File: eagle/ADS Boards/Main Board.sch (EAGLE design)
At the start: 14 parts

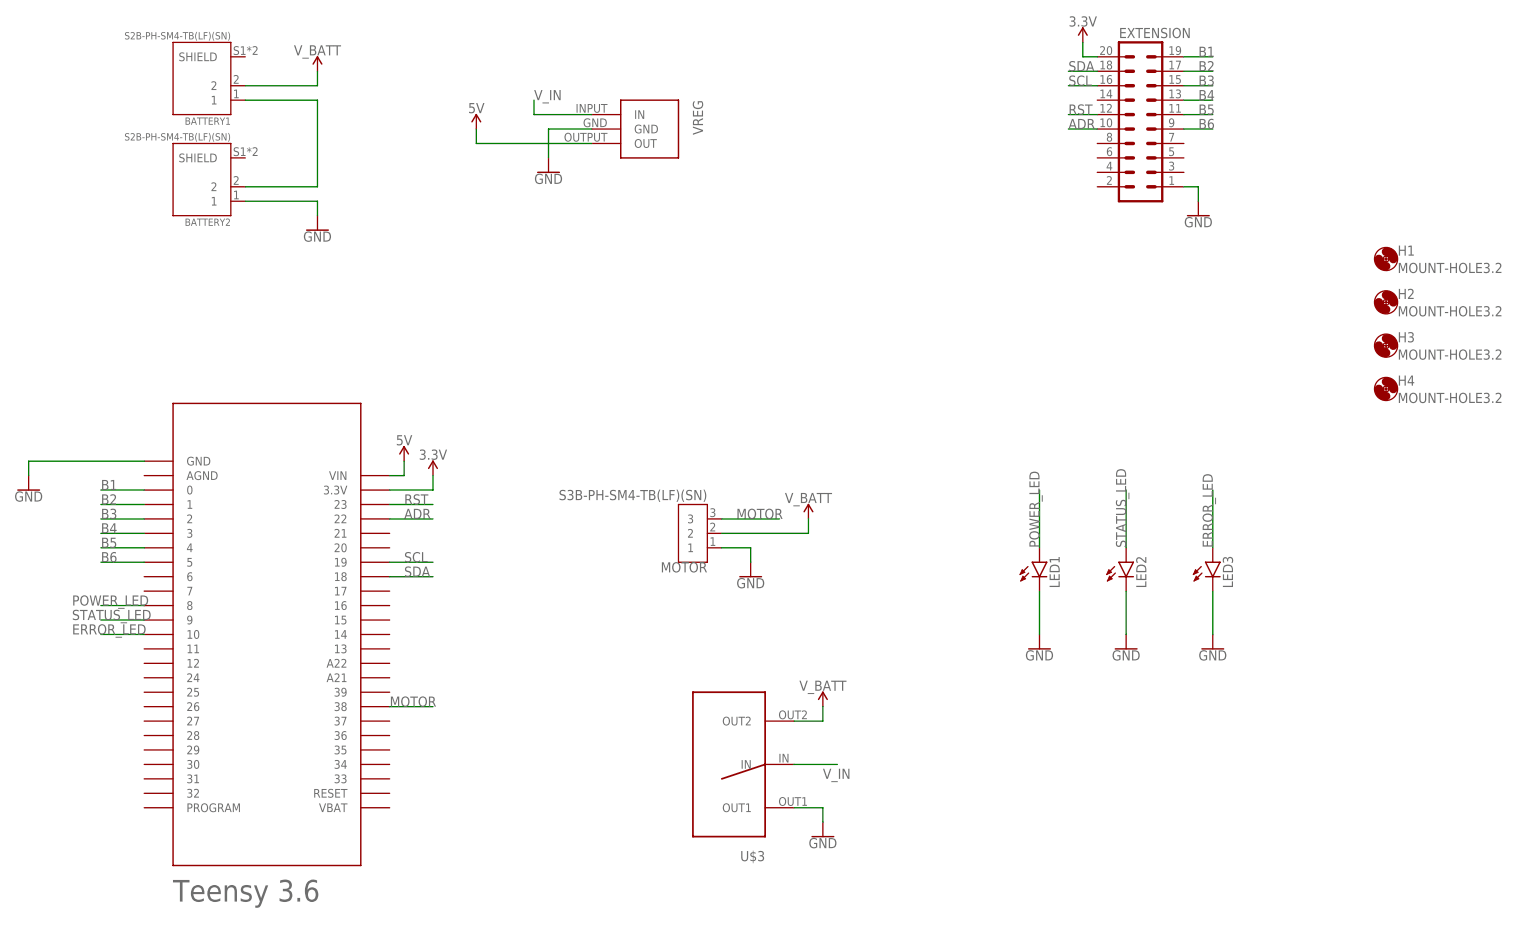
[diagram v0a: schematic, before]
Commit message: Finalized Boards, Gerbers, and DXF files.
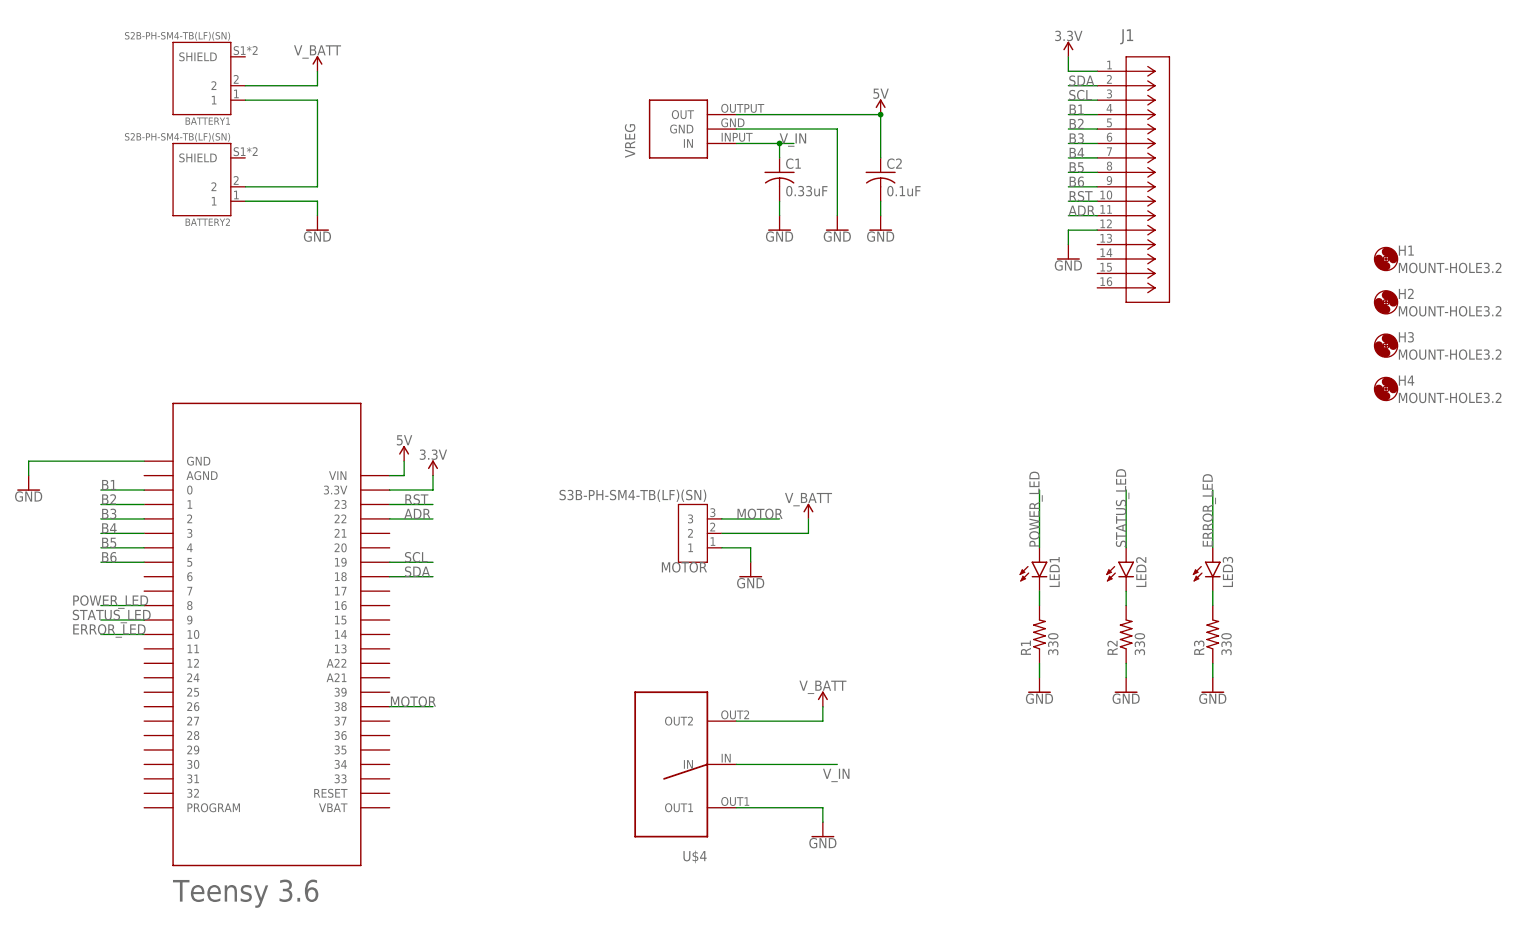
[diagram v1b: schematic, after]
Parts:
- removed EXTENSION: (no value), con-lstb:MA10-2
- removed U$3: SLIDE_SWITCH, ME433:SLIDE_SWITCH
- added C1: 0.33uF, resistor:C-USC0805
- added C2: 0.1uF, resistor:C-USC0805
- added J1: 62674-121121ALF, NUSTARS ADS Library:62674-121121ALF
- added R1, R2, R3: 330, resistor:R-US_R0805
- added U$4: SLIDE_SWITCH2, ME433:SLIDE_SWITCH2
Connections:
- new net N$1: LED1.C, R1.2
- new net N$3: LED2.C, R2.2
- new net N$4: LED3.C, R3.2
- net 3.3V: now also J1.11; no longer EXTENSION.20
- net 5V: now also C2.1
- net ADR: now also J1.1111; no longer EXTENSION.10
- net B1: now also J1.44; no longer EXTENSION.19
- net B2: now also J1.55; no longer EXTENSION.17
- net B3: now also J1.66; no longer EXTENSION.15
- net B4: now also J1.77; no longer EXTENSION.13
- net B5: now also J1.88; no longer EXTENSION.11
- net B6: now also J1.99; no longer EXTENSION.9
- net GND: now also C1.2, C2.2, J1.1212, R1.1, R2.1, R3.1, U$4.OUT1; no longer EXTENSION.1, LED1.C, LED2.C, LED3.C, U$3.OUT1
- net RST: now also J1.1010; no longer EXTENSION.12
- net SCL: now also J1.33; no longer EXTENSION.16
- net SDA: now also J1.22; no longer EXTENSION.18
- net V_BATT: now also U$4.OUT2; no longer U$3.OUT2
- net V_IN: now also C1.1, U$4.IN; no longer U$3.IN
